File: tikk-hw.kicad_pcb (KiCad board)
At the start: 4 copper layers, 18.1 x 39 mm, 116 parts, among them P6 ZX-SH1.0-4PWT, SW1 TS24CA, SW2 TS24CA, U1 IS31FL3731-QFLS2-TR, U2 LIS2DH12TR, U4 CP6208DTR(XBLW), U5 TMP102AIDRLR

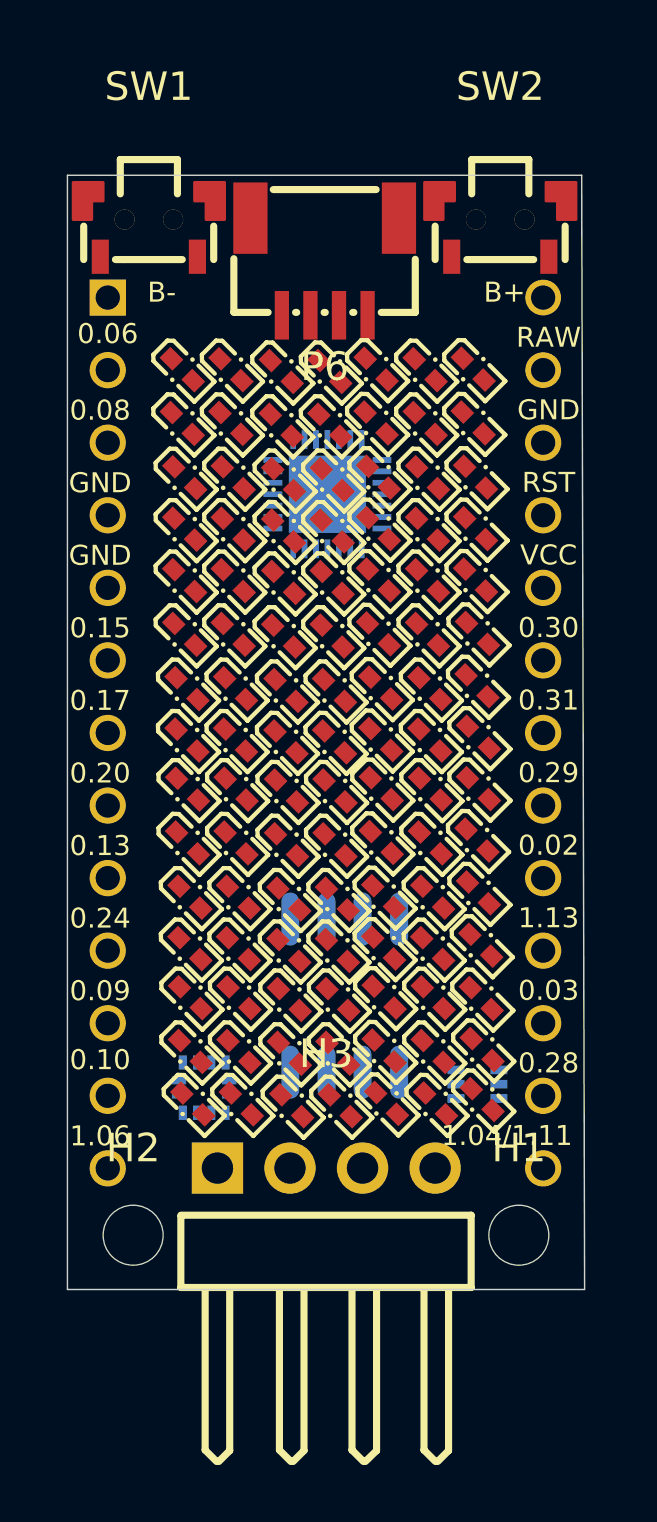
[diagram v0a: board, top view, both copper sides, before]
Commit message: initial placements all finished
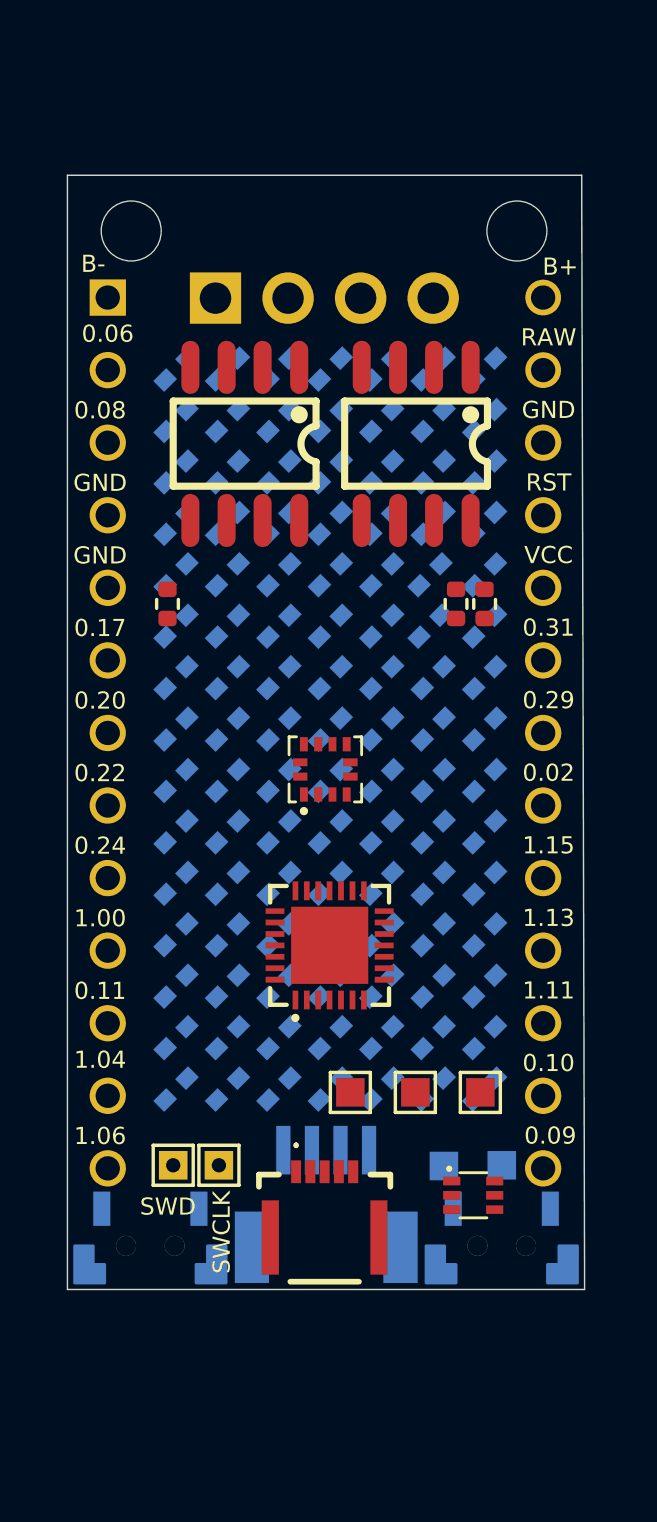
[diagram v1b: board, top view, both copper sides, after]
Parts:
- removed the LED1 at (169.1, 110.5)
- removed the LED1 at (169.2, 112.3)
- removed the LED1 at (169.0, 97.8)
- removed the LED1 at (169.0, 108.7)
- removed the LED1 at (169.2, 114.2)
- removed the LED1 at (169.0, 99.6)
- removed the LED1 at (169.1, 106.9)
- removed the LED1 at (169.1, 101.4)
- removed the LED1 at (169.1, 105.1)
- removed the LED1 at (169.0, 96.0)
- removed the LED1 at (168.9, 94.1)
- removed the LED1 at (169.0, 103.3)
- removed the LED1 at (168.9, 92.2)
- removed the LED1 at (169.2, 116.0)
- removed the LED2 at (167.3, 99.6)
- removed the LED2 at (167.4, 103.4)
- removed the LED2 at (167.3, 97.8)
- removed the LED2 at (167.5, 110.7)
- removed the LED2 at (167.4, 106.9)
- removed the LED2 at (167.4, 105.2)
- removed the LED2 at (167.2, 94.1)
- removed the LED2 at (167.5, 114.2)
- removed the LED2 at (167.3, 101.5)
- removed the LED2 at (167.3, 96.0)
- removed the LED2 at (167.5, 116.1)
- removed the LED2 at (169.2, 117.8)
- removed the LED2 at (167.4, 108.8)
- removed the LED2 at (167.6, 117.9)
- removed the LED2 at (167.5, 112.5)
- removed the LED2 at (167.2, 92.2)
- removed the LED3 at (165.7, 106.9)
- removed the LED3 at (165.8, 110.7)
- removed the LED3 at (165.7, 103.3)
- removed the LED3 at (165.6, 101.5)
- removed the LED3 at (165.7, 105.2)
- removed the LED3 at (165.5, 94.1)
- removed the LED3 at (165.7, 108.8)
- removed the LED3 at (165.6, 96.0)
- removed the LED3 at (165.8, 116.0)
- removed the LED3 at (165.9, 117.9)
- removed the LED3 at (165.8, 114.2)
- removed the LED3 at (165.5, 92.2)
- removed the LED3 at (165.6, 99.6)
- removed the LED3 at (165.6, 97.8)
- removed the LED3 at (165.8, 112.5)
- removed the LED4 at (164.1, 103.4)
- removed the LED4 at (164.2, 110.7)
- removed the LED4 at (164.0, 101.5)
- removed the LED4 at (164.0, 97.8)
- removed the LED4 at (164.0, 96.0)
- removed the LED4 at (164.1, 107.0)
- removed the LED4 at (164.2, 116.1)
- removed the LED4 at (164.2, 112.5)
- removed the LED4 at (163.9, 92.3)
- removed the LED4 at (164.0, 99.7)
- removed the LED4 at (164.2, 118.0)
- removed the LED4 at (164.2, 114.2)
- removed the LED4 at (163.9, 94.2)
- removed the LED4 at (164.1, 105.2)
- removed the LED4 at (164.1, 108.8)
- removed the LED5 at (162.3, 97.8)
- removed the LED5 at (162.4, 108.8)
- removed the LED5 at (162.3, 101.5)
- removed the LED5 at (162.5, 116.1)
- removed the LED5 at (162.4, 110.7)
- removed the LED5 at (162.4, 112.5)
- removed the LED5 at (162.6, 118.0)
- removed the LED5 at (162.2, 92.3)
- removed the LED5 at (162.3, 103.4)
- removed the LED5 at (162.3, 99.7)
- removed the LED5 at (162.3, 96.0)
- removed the LED5 at (162.5, 114.2)
- removed the LED5 at (162.4, 107.0)
- removed the LED5 at (162.3, 105.2)
- removed the LED5 at (162.2, 94.2)
- removed the LED6 at (160.6, 103.4)
- removed the LED6 at (160.7, 116.1)
- removed the LED6 at (160.5, 101.5)
- removed the LED6 at (160.8, 117.9)
- removed the LED6 at (160.5, 99.6)
- removed the LED6 at (160.6, 108.8)
- removed the LED6 at (160.6, 106.9)
- removed the LED6 at (160.7, 110.7)
- removed the LED6 at (160.5, 97.8)
- removed the LED6 at (160.4, 92.2)
- removed the LED6 at (160.7, 112.5)
- removed the LED6 at (160.7, 114.2)
- removed the LED6 at (160.4, 94.1)
- removed the LED6 at (160.6, 105.2)
- removed the LED6 at (160.5, 96.0)
- removed the LED7 at (159.0, 114.2)
- removed the LED7 at (159.0, 112.5)
- removed the LED7 at (158.9, 108.8)
- removed the LED7 at (158.9, 103.4)
- removed the LED7 at (158.9, 106.9)
- removed the LED7 at (158.8, 101.5)
- removed the LED7 at (158.8, 96.0)
- removed the LED7 at (158.9, 105.2)
- removed the LED7 at (158.8, 97.8)
- removed the LED7 at (158.7, 94.1)
- removed the LED7 at (159.0, 110.7)
- removed the LED7 at (158.7, 92.2)
- removed the LED7 at (158.8, 99.6)
- removed the LED7 at (159.0, 116.1)
- removed the LED7 at (159.1, 117.9)
- added J1: 51281-0598, easyeda2kicad:512810598, F.Cu at (163.7, 122.2)
- added LED1: F.0402.00003/P2-0402R1TS2-045T-001, easyeda2kicad:LED0402-RD, B.Cu at (169.3, 92.2)
- added LED10: F.0402.00003/P2-0402R1TS2-045T-001, easyeda2kicad:LED0402-RD, B.Cu at (165.7, 94.0)
- added LED100: F.0402.00003/P2-0402R1TS2-045T-001, easyeda2kicad:LED0402-RD, B.Cu at (167.5, 110.2)
- added LED101: F.0402.00003/P2-0402R1TS2-045T-001, easyeda2kicad:LED0402-RD, B.Cu at (165.7, 110.2)
- added LED102: F.0402.00003/P2-0402R1TS2-045T-001, easyeda2kicad:LED0402-RD, B.Cu at (163.9, 110.2)
- added LED103: F.0402.00003/P2-0402R1TS2-045T-001, easyeda2kicad:LED0402-RD, B.Cu at (162.1, 110.2)
- added LED104: F.0402.00003/P2-0402R1TS2-045T-001, easyeda2kicad:LED0402-RD, B.Cu at (160.3, 110.2)
- added LED105: F.0402.00003/P2-0402R1TS2-045T-001, easyeda2kicad:LED0402-RD, B.Cu at (158.5, 110.2)
- added LED11: F.0402.00003/P2-0402R1TS2-045T-001, easyeda2kicad:LED0402-RD, B.Cu at (163.9, 94.0)
- added LED12: F.0402.00003/P2-0402R1TS2-045T-001, easyeda2kicad:LED0402-RD, B.Cu at (162.1, 94.0)
- added LED13: F.0402.00003/P2-0402R1TS2-045T-001, easyeda2kicad:LED0402-RD, B.Cu at (160.3, 94.0)
- added LED14: F.0402.00003/P2-0402R1TS2-045T-001, easyeda2kicad:LED0402-RD, B.Cu at (158.5, 94.0)
- added LED15: F.0402.00003/P2-0402R1TS2-045T-001, easyeda2kicad:LED0402-RD, B.Cu at (169.3, 95.8)
- added LED16: F.0402.00003/P2-0402R1TS2-045T-001, easyeda2kicad:LED0402-RD, B.Cu at (167.5, 95.8)
- added LED17: F.0402.00003/P2-0402R1TS2-045T-001, easyeda2kicad:LED0402-RD, B.Cu at (165.7, 95.8)
- added LED18: F.0402.00003/P2-0402R1TS2-045T-001, easyeda2kicad:LED0402-RD, B.Cu at (163.9, 95.8)
- added LED19: F.0402.00003/P2-0402R1TS2-045T-001, easyeda2kicad:LED0402-RD, B.Cu at (162.1, 95.8)
- added LED2: F.0402.00003/P2-0402R1TS2-045T-001, easyeda2kicad:LED0402-RD, B.Cu at (167.5, 92.2)
- added LED20: F.0402.00003/P2-0402R1TS2-045T-001, easyeda2kicad:LED0402-RD, B.Cu at (160.3, 95.8)
- added LED21: F.0402.00003/P2-0402R1TS2-045T-001, easyeda2kicad:LED0402-RD, B.Cu at (158.5, 95.8)
- added LED22: F.0402.00003/P2-0402R1TS2-045T-001, easyeda2kicad:LED0402-RD, B.Cu at (169.3, 97.6)
- added LED23: F.0402.00003/P2-0402R1TS2-045T-001, easyeda2kicad:LED0402-RD, B.Cu at (167.5, 97.6)
- added LED24: F.0402.00003/P2-0402R1TS2-045T-001, easyeda2kicad:LED0402-RD, B.Cu at (165.7, 97.6)
- added LED25: F.0402.00003/P2-0402R1TS2-045T-001, easyeda2kicad:LED0402-RD, B.Cu at (163.9, 97.6)
- added LED26: F.0402.00003/P2-0402R1TS2-045T-001, easyeda2kicad:LED0402-RD, B.Cu at (162.1, 97.6)
- added LED27: F.0402.00003/P2-0402R1TS2-045T-001, easyeda2kicad:LED0402-RD, B.Cu at (160.3, 97.6)
- added LED28: F.0402.00003/P2-0402R1TS2-045T-001, easyeda2kicad:LED0402-RD, B.Cu at (158.5, 97.6)
- added LED29: F.0402.00003/P2-0402R1TS2-045T-001, easyeda2kicad:LED0402-RD, B.Cu at (169.3, 99.4)
- added LED3: F.0402.00003/P2-0402R1TS2-045T-001, easyeda2kicad:LED0402-RD, B.Cu at (165.7, 92.2)
- added LED30: F.0402.00003/P2-0402R1TS2-045T-001, easyeda2kicad:LED0402-RD, B.Cu at (167.4, 99.4)
- added LED31: F.0402.00003/P2-0402R1TS2-045T-001, easyeda2kicad:LED0402-RD, B.Cu at (165.7, 99.4)
- added LED32: F.0402.00003/P2-0402R1TS2-045T-001, easyeda2kicad:LED0402-RD, B.Cu at (163.9, 99.4)
- added LED33: F.0402.00003/P2-0402R1TS2-045T-001, easyeda2kicad:LED0402-RD, B.Cu at (162.1, 99.4)
- added LED34: F.0402.00003/P2-0402R1TS2-045T-001, easyeda2kicad:LED0402-RD, B.Cu at (160.3, 99.4)
- added LED35: F.0402.00003/P2-0402R1TS2-045T-001, easyeda2kicad:LED0402-RD, B.Cu at (158.5, 99.4)
- added LED36: F.0402.00003/P2-0402R1TS2-045T-001, easyeda2kicad:LED0402-RD, B.Cu at (169.3, 108.4)
- added LED37: F.0402.00003/P2-0402R1TS2-045T-001, easyeda2kicad:LED0402-RD, B.Cu at (167.5, 108.4)
- added LED38: F.0402.00003/P2-0402R1TS2-045T-001, easyeda2kicad:LED0402-RD, B.Cu at (165.7, 108.4)
- added LED39: F.0402.00003/P2-0402R1TS2-045T-001, easyeda2kicad:LED0402-RD, B.Cu at (163.9, 108.4)
- added LED4: F.0402.00003/P2-0402R1TS2-045T-001, easyeda2kicad:LED0402-RD, B.Cu at (163.9, 92.2)
- added LED40: F.0402.00003/P2-0402R1TS2-045T-001, easyeda2kicad:LED0402-RD, B.Cu at (162.1, 108.4)
- added LED41: F.0402.00003/P2-0402R1TS2-045T-001, easyeda2kicad:LED0402-RD, B.Cu at (160.3, 108.4)
- added LED42: F.0402.00003/P2-0402R1TS2-045T-001, easyeda2kicad:LED0402-RD, B.Cu at (158.5, 108.4)
- added LED43: F.0402.00003/P2-0402R1TS2-045T-001, easyeda2kicad:LED0402-RD, B.Cu at (169.3, 106.6)
- added LED44: F.0402.00003/P2-0402R1TS2-045T-001, easyeda2kicad:LED0402-RD, B.Cu at (167.5, 106.6)
- added LED45: F.0402.00003/P2-0402R1TS2-045T-001, easyeda2kicad:LED0402-RD, B.Cu at (165.7, 106.6)
- added LED46: F.0402.00003/P2-0402R1TS2-045T-001, easyeda2kicad:LED0402-RD, B.Cu at (163.9, 106.6)
- added LED47: F.0402.00003/P2-0402R1TS2-045T-001, easyeda2kicad:LED0402-RD, B.Cu at (162.1, 106.6)
- added LED48: F.0402.00003/P2-0402R1TS2-045T-001, easyeda2kicad:LED0402-RD, B.Cu at (160.3, 106.6)
- added LED49: F.0402.00003/P2-0402R1TS2-045T-001, easyeda2kicad:LED0402-RD, B.Cu at (158.5, 106.6)
- added LED5: F.0402.00003/P2-0402R1TS2-045T-001, easyeda2kicad:LED0402-RD, B.Cu at (162.1, 92.2)
- added LED50: F.0402.00003/P2-0402R1TS2-045T-001, easyeda2kicad:LED0402-RD, B.Cu at (169.3, 104.8)
- added LED51: F.0402.00003/P2-0402R1TS2-045T-001, easyeda2kicad:LED0402-RD, B.Cu at (167.5, 104.8)
- added LED52: F.0402.00003/P2-0402R1TS2-045T-001, easyeda2kicad:LED0402-RD, B.Cu at (165.7, 104.8)
- added LED53: F.0402.00003/P2-0402R1TS2-045T-001, easyeda2kicad:LED0402-RD, B.Cu at (163.9, 104.8)
- added LED54: F.0402.00003/P2-0402R1TS2-045T-001, easyeda2kicad:LED0402-RD, B.Cu at (162.1, 104.8)
- added LED55: F.0402.00003/P2-0402R1TS2-045T-001, easyeda2kicad:LED0402-RD, B.Cu at (160.3, 104.8)
- added LED56: F.0402.00003/P2-0402R1TS2-045T-001, easyeda2kicad:LED0402-RD, B.Cu at (158.5, 104.8)
- added LED57: F.0402.00003/P2-0402R1TS2-045T-001, easyeda2kicad:LED0402-RD, B.Cu at (169.3, 103.0)
- added LED58: F.0402.00003/P2-0402R1TS2-045T-001, easyeda2kicad:LED0402-RD, B.Cu at (167.5, 103.0)
- added LED59: F.0402.00003/P2-0402R1TS2-045T-001, easyeda2kicad:LED0402-RD, B.Cu at (165.7, 103.0)
- added LED6: F.0402.00003/P2-0402R1TS2-045T-001, easyeda2kicad:LED0402-RD, B.Cu at (160.3, 92.2)
- added LED60: F.0402.00003/P2-0402R1TS2-045T-001, easyeda2kicad:LED0402-RD, B.Cu at (163.9, 103.0)
- added LED61: F.0402.00003/P2-0402R1TS2-045T-001, easyeda2kicad:LED0402-RD, B.Cu at (162.1, 103.0)
- added LED62: F.0402.00003/P2-0402R1TS2-045T-001, easyeda2kicad:LED0402-RD, B.Cu at (160.3, 103.0)
- added LED63: F.0402.00003/P2-0402R1TS2-045T-001, easyeda2kicad:LED0402-RD, B.Cu at (158.5, 103.0)
- added LED64: F.0402.00003/P2-0402R1TS2-045T-001, easyeda2kicad:LED0402-RD, B.Cu at (169.3, 101.2)
- added LED65: F.0402.00003/P2-0402R1TS2-045T-001, easyeda2kicad:LED0402-RD, B.Cu at (167.4, 101.2)
- added LED66: F.0402.00003/P2-0402R1TS2-045T-001, easyeda2kicad:LED0402-RD, B.Cu at (165.7, 101.2)
- added LED67: F.0402.00003/P2-0402R1TS2-045T-001, easyeda2kicad:LED0402-RD, B.Cu at (163.9, 101.2)
- added LED68: F.0402.00003/P2-0402R1TS2-045T-001, easyeda2kicad:LED0402-RD, B.Cu at (162.1, 101.2)
- added LED69: F.0402.00003/P2-0402R1TS2-045T-001, easyeda2kicad:LED0402-RD, B.Cu at (160.3, 101.2)
- added LED7: F.0402.00003/P2-0402R1TS2-045T-001, easyeda2kicad:LED0402-RD, B.Cu at (158.5, 92.2)
- added LED70: F.0402.00003/P2-0402R1TS2-045T-001, easyeda2kicad:LED0402-RD, B.Cu at (158.5, 101.2)
- added LED71: F.0402.00003/P2-0402R1TS2-045T-001, easyeda2kicad:LED0402-RD, B.Cu at (169.3, 117.4)
- added LED72: F.0402.00003/P2-0402R1TS2-045T-001, easyeda2kicad:LED0402-RD, B.Cu at (167.5, 117.4)
- added LED73: F.0402.00003/P2-0402R1TS2-045T-001, easyeda2kicad:LED0402-RD, B.Cu at (165.7, 117.4)
- added LED74: F.0402.00003/P2-0402R1TS2-045T-001, easyeda2kicad:LED0402-RD, B.Cu at (163.9, 117.4)
- added LED75: F.0402.00003/P2-0402R1TS2-045T-001, easyeda2kicad:LED0402-RD, B.Cu at (162.1, 117.4)
- added LED76: F.0402.00003/P2-0402R1TS2-045T-001, easyeda2kicad:LED0402-RD, B.Cu at (160.3, 117.4)
- added LED77: F.0402.00003/P2-0402R1TS2-045T-001, easyeda2kicad:LED0402-RD, B.Cu at (158.5, 117.4)
- added LED78: F.0402.00003/P2-0402R1TS2-045T-001, easyeda2kicad:LED0402-RD, B.Cu at (169.3, 115.6)
- added LED79: F.0402.00003/P2-0402R1TS2-045T-001, easyeda2kicad:LED0402-RD, B.Cu at (167.5, 115.6)
- added LED8: F.0402.00003/P2-0402R1TS2-045T-001, easyeda2kicad:LED0402-RD, B.Cu at (169.3, 94.0)
- added LED80: F.0402.00003/P2-0402R1TS2-045T-001, easyeda2kicad:LED0402-RD, B.Cu at (165.7, 115.6)
- added LED81: F.0402.00003/P2-0402R1TS2-045T-001, easyeda2kicad:LED0402-RD, B.Cu at (163.9, 115.6)
- added LED82: F.0402.00003/P2-0402R1TS2-045T-001, easyeda2kicad:LED0402-RD, B.Cu at (162.1, 115.6)
- added LED83: F.0402.00003/P2-0402R1TS2-045T-001, easyeda2kicad:LED0402-RD, B.Cu at (160.3, 115.6)
- added LED84: F.0402.00003/P2-0402R1TS2-045T-001, easyeda2kicad:LED0402-RD, B.Cu at (158.5, 115.6)
- added LED85: F.0402.00003/P2-0402R1TS2-045T-001, easyeda2kicad:LED0402-RD, B.Cu at (169.3, 113.8)
- added LED86: F.0402.00003/P2-0402R1TS2-045T-001, easyeda2kicad:LED0402-RD, B.Cu at (167.5, 113.8)
- added LED87: F.0402.00003/P2-0402R1TS2-045T-001, easyeda2kicad:LED0402-RD, B.Cu at (165.7, 113.8)
- added LED88: F.0402.00003/P2-0402R1TS2-045T-001, easyeda2kicad:LED0402-RD, B.Cu at (163.9, 113.8)
- added LED89: F.0402.00003/P2-0402R1TS2-045T-001, easyeda2kicad:LED0402-RD, B.Cu at (162.1, 113.8)
- added LED9: F.0402.00003/P2-0402R1TS2-045T-001, easyeda2kicad:LED0402-RD, B.Cu at (167.5, 94.0)
- added LED90: F.0402.00003/P2-0402R1TS2-045T-001, easyeda2kicad:LED0402-RD, B.Cu at (160.3, 113.8)
- added LED91: F.0402.00003/P2-0402R1TS2-045T-001, easyeda2kicad:LED0402-RD, B.Cu at (158.5, 113.8)
- added LED92: F.0402.00003/P2-0402R1TS2-045T-001, easyeda2kicad:LED0402-RD, B.Cu at (169.3, 112.0)
- added LED93: F.0402.00003/P2-0402R1TS2-045T-001, easyeda2kicad:LED0402-RD, B.Cu at (167.5, 112.0)
- added LED94: F.0402.00003/P2-0402R1TS2-045T-001, easyeda2kicad:LED0402-RD, B.Cu at (165.7, 112.0)
- added LED95: F.0402.00003/P2-0402R1TS2-045T-001, easyeda2kicad:LED0402-RD, B.Cu at (163.9, 112.0)
- added LED96: F.0402.00003/P2-0402R1TS2-045T-001, easyeda2kicad:LED0402-RD, B.Cu at (162.1, 112.0)
- added LED97: F.0402.00003/P2-0402R1TS2-045T-001, easyeda2kicad:LED0402-RD, B.Cu at (160.3, 112.0)
- added LED98: F.0402.00003/P2-0402R1TS2-045T-001, easyeda2kicad:LED0402-RD, B.Cu at (158.5, 112.0)
- added LED99: F.0402.00003/P2-0402R1TS2-045T-001, easyeda2kicad:LED0402-RD, B.Cu at (169.3, 110.2)
- added R1: 100K, Resistor_SMD:R_0402_1005Metric, F.Cu at (168.3, 100.4)
- added R1: 100K, Resistor_SMD:R_0402_1005Metric, F.Cu at (158.2, 100.4)
- added R2: 100K, Resistor_SMD:R_0402_1005Metric, F.Cu at (169.3, 100.4)
- added TP1: NC1, TestPoint:TestPoint_Pad_1.0x1.0mm, F.Cu at (164.6, 117.5)
- added TP2: NFC1, TestPoint:TestPoint_Pad_1.0x1.0mm, B.Cu at (167.9, 120.1)
- added TP3: NC2, TestPoint:TestPoint_Pad_1.0x1.0mm, F.Cu at (169.2, 117.5)
- added TP4: NC3, TestPoint:TestPoint_Pad_1.0x1.0mm, F.Cu at (166.9, 117.5)
- added TP5: NFC2, TestPoint:TestPoint_Pad_1.0x1.0mm, B.Cu at (169.9, 120.1)
- added TP6: SWCLK, TestPoint:TestPoint_THTPad_1.0x1.0mm_Drill0.5mm, F.Cu at (160.0, 120.1)
- added TP7: SWDIO, TestPoint:TestPoint_THTPad_1.0x1.0mm_Drill0.5mm, F.Cu at (158.4, 120.1)
- added U6: CP6208DTR(XBLW), easyeda2kicad:SOP-8_L4.9-W3.9-P1.27-LS6.0-BL, F.Cu at (160.9, 94.8)
- H1, H2, H3, P6, SW1, SW2: moved to B.Cu
- U1, U2, U4, U5: moved to F.Cu
- U3: renamed from U4; value CP6208DTR(XBLW) -> Tenstar nRF52840
- moved SW1 35.3 mm to (157.6, 122.6)
- moved SW2 35.3 mm to (169.9, 122.6)
- moved H1 35.1 mm to (170.4, 87.4)
- moved H2 35.1 mm to (156.9, 87.4)
- moved P6 32.6 mm to (163.8, 121.2)
- moved H3 30.4 mm to (163.7, 89.7)
- moved U4 19.5 mm to (166.9, 94.8)
- moved U1 15.8 mm to (163.9, 112.4), turned to 0 degrees
- moved U2 11.9 mm to (163.7, 106.2), turned to 0 degrees
- moved U5 3.89 mm to (168.9, 121.1)
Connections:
- H3 pad 1: unconnected-(H3-Pad1) -> Net-(U6-Bout)
- H3 pad 2: unconnected-(H3-Pad2) -> Net-(U6-Aout)
- H3 pad 3: unconnected-(H3-Pad3) -> Net-(U4-Bout)
- H3 pad 4: unconnected-(H3-Pad4) -> Net-(U4-Aout)
- SW1 pad 3: unconnected-(SW1-Pad3) -> GND
- SW1 pad 4: unconnected-(SW1-Pad4) -> RESET
- U3 pad 1: unconnected-(U4-Vcc-Pad1) -> VBAT
- U3 pad 10: (no net) -> /P1.11
- U3 pad 11: (no net) -> /P0.10
- U3 pad 12: (no net) -> /P0.09
- U3 pad 13: (no net) -> MOTOR1-A
- U3 pad 14: (no net) -> MOTOR1-B
- U3 pad 15: (no net) -> GND
- U3 pad 16: (no net) -> GND
- U3 pad 17: (no net) -> MOTOR2-A
- U3 pad 18: (no net) -> MOTOR2-B
- U3 pad 19: (no net) -> /P0.22
- U3 pad 2: unconnected-(U4-Bout-Pad2) -> GND
- U3 pad 20: (no net) -> /P0.24
- U3 pad 21: (no net) -> /P1.00
- U3 pad 22: (no net) -> /P0.13
- U3 pad 23: (no net) -> SCL
- U3 pad 24: (no net) -> SDA
- U3 pad 3: unconnected-(U4-Aout-Pad3) -> RESET
- U3 pad 4: unconnected-(U4-GND-Pad4) -> EXT_VCC
- U3 pad 5: unconnected-(U4-Bin-Pad5) -> BATTERY-V
- U3 pad 6: unconnected-(U4-NC-Pad6) -> /P0.29
- U3 pad 7: unconnected-(U4-GND-Pad7) -> /P0.02
- U3 pad 8: unconnected-(U4-Ain-Pad8) -> /P1.15
- U3 pad 9: (no net) -> /P1.13
- U4 pad 2: unconnected-(U4-Bout-Pad2) -> Net-(U4-Bout)
- U4 pad 3: unconnected-(U4-Aout-Pad3) -> Net-(U4-Aout)
- U4 pad 5: unconnected-(U4-Bin-Pad5) -> MOTOR2-B
- U4 pad 8: unconnected-(U4-Ain-Pad8) -> MOTOR2-A
- U5 pad 1: unconnected-(U5-SCL-Pad1) -> SCL
- U5 pad 2: unconnected-(U5-GND-Pad2) -> GND
- U5 pad 3: unconnected-(U5-ALERT-Pad3) -> TMP102_ALERT
- U5 pad 4: unconnected-(U5-ADD0-Pad4) -> GND
- U5 pad 5: unconnected-(U5-V+-Pad5) -> EXT_VCC
- U5 pad 6: unconnected-(U5-SDA-Pad6) -> SDA
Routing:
- added copper zone on In2.Cu, net EXT_VCC
- added copper zone on In1.Cu, net GND
- added copper zone on In2.Cu, net VBAT
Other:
- board text added: "1"
- board text added: "2"
- board text added: "C"
- board text added: "D"
- board text added: "SWCLK"
- board text added: "SWD"
- board text removed: "B+"
- board text removed: "B-"
- board text removed: "U4"
